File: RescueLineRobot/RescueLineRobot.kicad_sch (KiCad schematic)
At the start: 11 parts, among them J1 Conn_01x11, J2 Switch, J3 Motor 1, J4 Motor 2, J5 Convertidor, J6 Laser 1, J7 Laser 2, J8 Laser 3, J9 Bateria, U1 ROB-14450, U2 ESP32-DEVKIT-V1

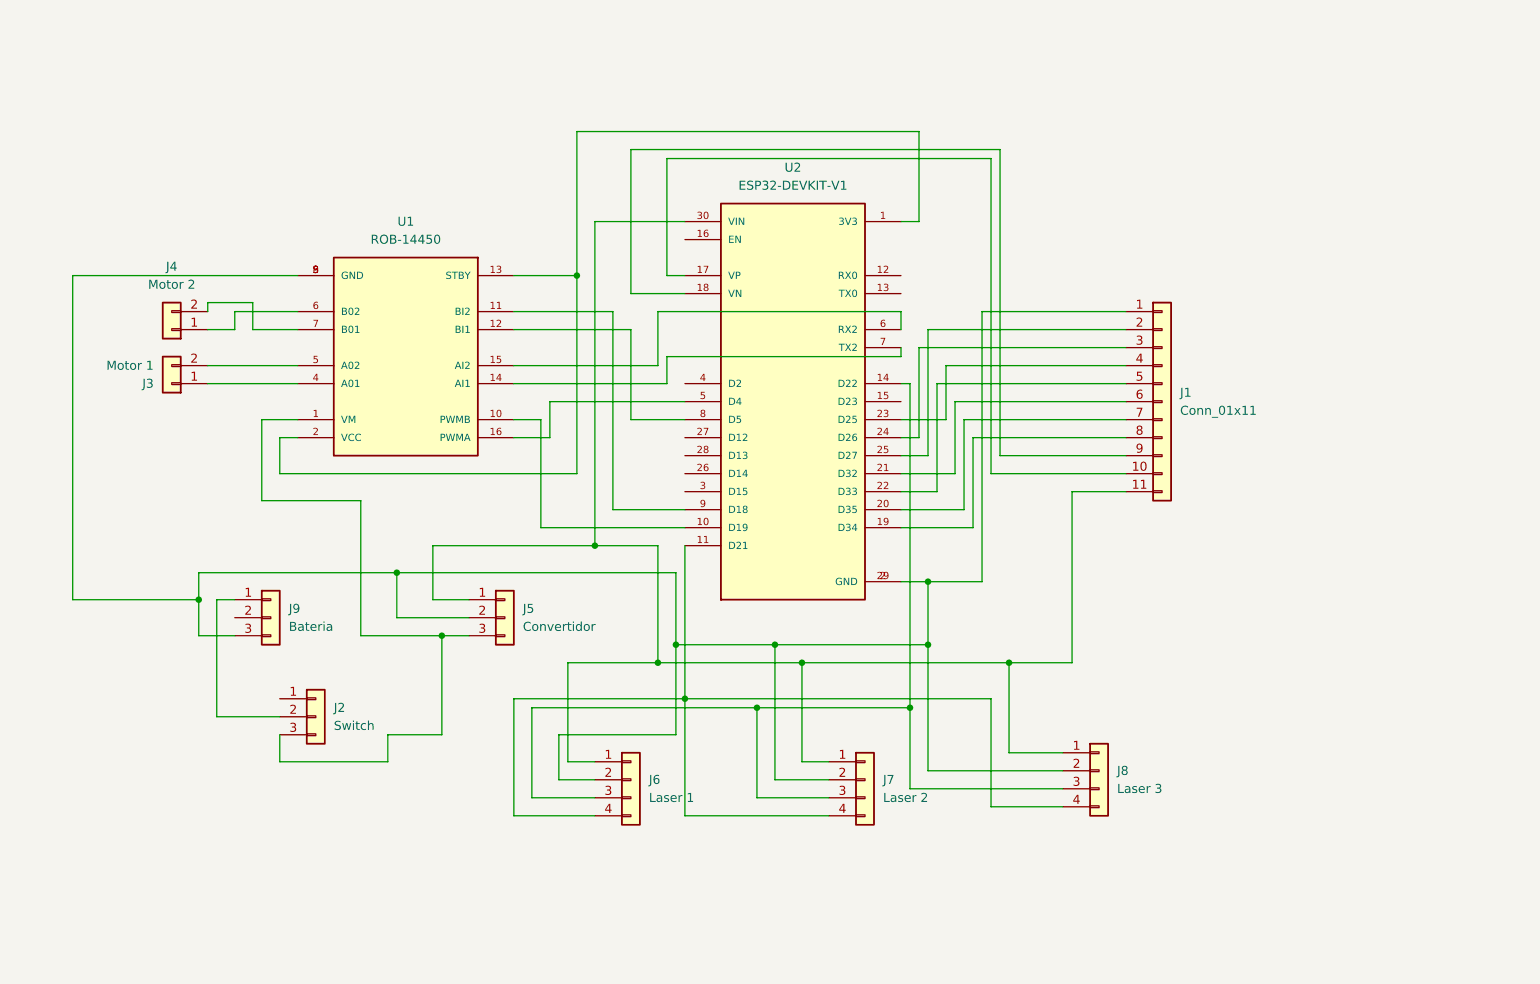
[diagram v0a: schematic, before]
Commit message: Boton y encoders
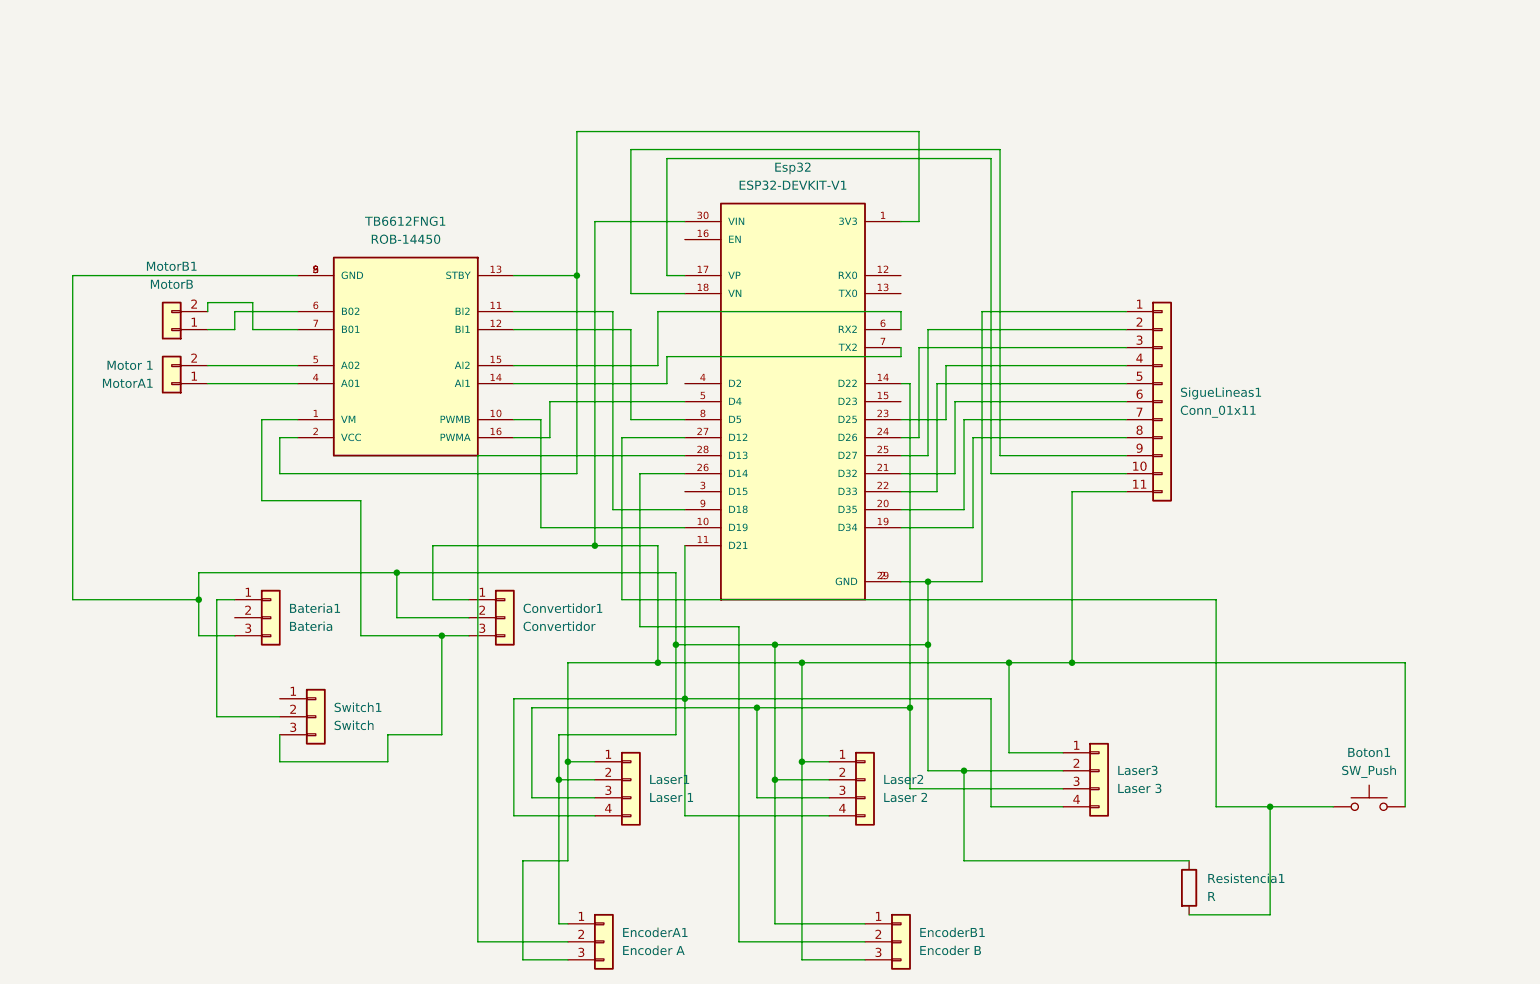
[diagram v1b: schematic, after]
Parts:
- added Boton1: SW_Push, Button_Switch_THT:SW_PUSH-12mm, symbol Switch:SW_Push
- added EncoderA1: Encoder A, Connector_JST:JST_XA_B03B-XASK-1_1x03_P2.50mm_Vertical, symbol Connector_Generic:Conn_01x03
- added EncoderB1: Encoder B, Connector_JST:JST_XA_B03B-XASK-1_1x03_P2.50mm_Vertical, symbol Connector_Generic:Conn_01x03
- added Resistencia1: R, Resistor_THT:R_Axial_DIN0617_L17.0mm_D6.0mm_P25.40mm_Horizontal, symbol Device:R
- MotorB1: renamed from J4; value Motor 2 -> MotorB
- renumbered J9 to Bateria1, J5 to Convertidor1, U2 to Esp32, J6 to Laser1, J7 to Laser2, J8 to Laser3, J3 to MotorA1, J1 to SigueLineas1, J2 to Switch1, U1 to TB6612FNG1
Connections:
- net at Convertidor1.1 (Pin_1), Esp32.30 (VIN), Laser1.1 (Pin_1)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: now also Boton1.2, EncoderA1.3 (Pin_3), EncoderB1.3 (Pin_3)
- net at Bateria1.3 (Pin_3), Convertidor1.2 (Pin_2), Esp32.2 (GND)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: now also EncoderA1.1 (Pin_1), EncoderB1.1 (Pin_1), Resistencia1.1
- net at Esp32.26 (D14): now also EncoderB1.2 (Pin_2)
- net at Esp32.27 (D12): now also Boton1.1, Resistencia1.2
- net at Esp32.28 (D13): now also EncoderA1.2 (Pin_2)

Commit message: Estamos Casi
Están todas las rutas hechas, todos los puertos necesarios, sólo falta nombrar al robot y poner gráficas
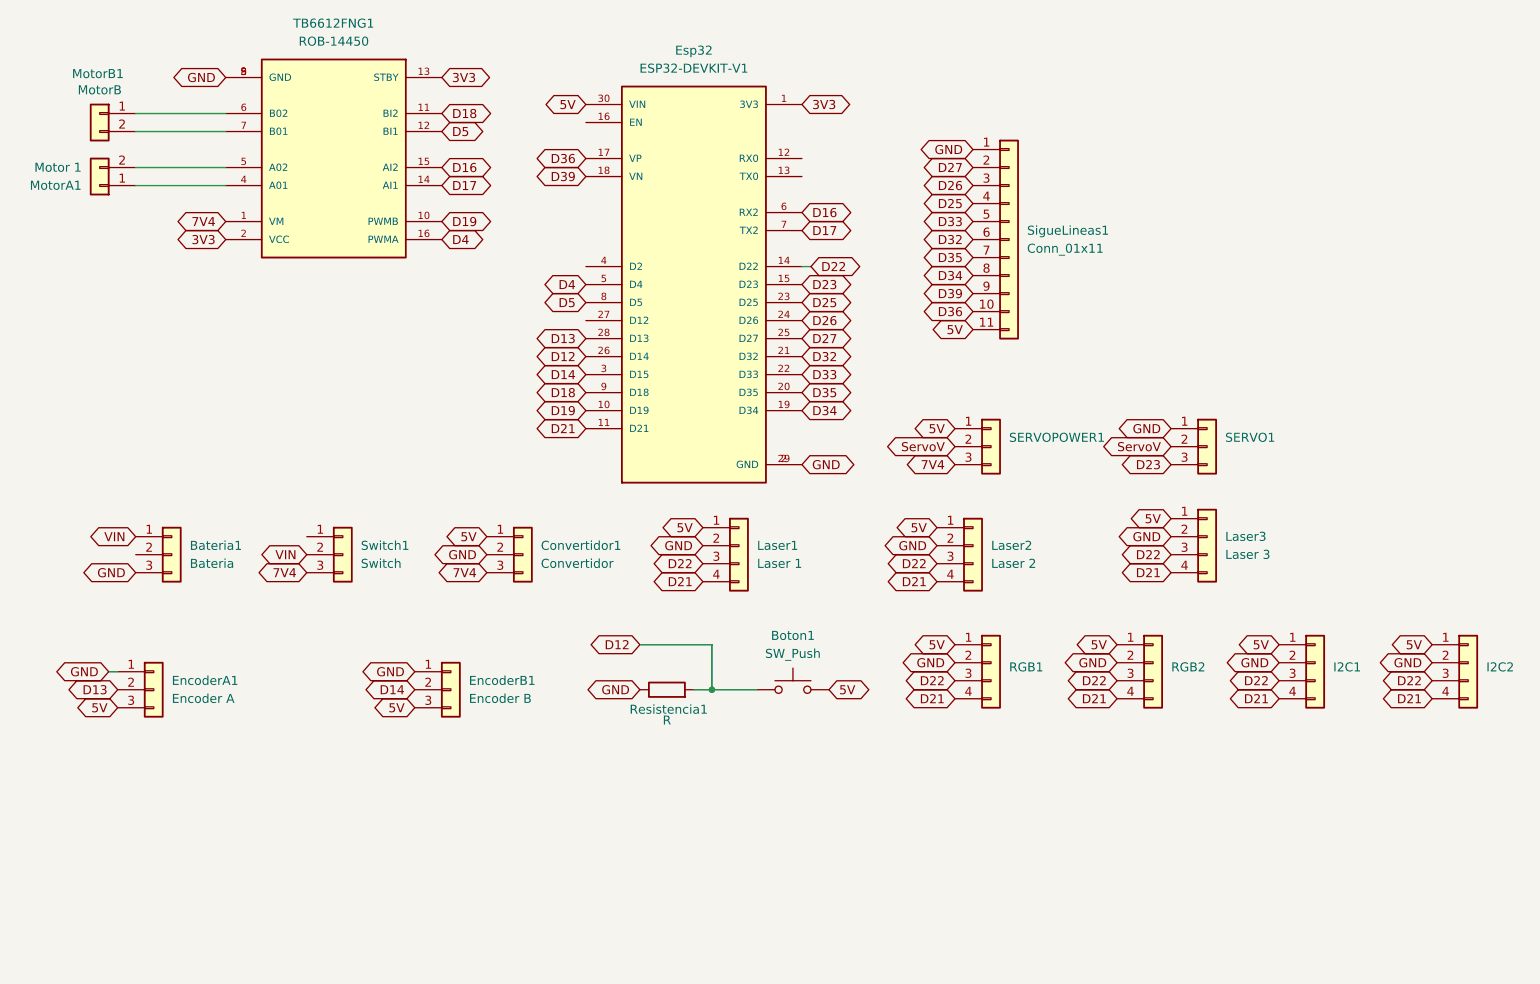
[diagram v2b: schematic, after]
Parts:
- added I2C1, I2C2, RGB1, RGB2: ~, Connector_JST:JST_XH_B4B-XH-A_1x04_P2.50mm_Vertical, symbol Connector_Generic:Conn_01x04
- added SERVO1: Conn_01x03, Connector_JST:JST_XH_B3B-XH-A_1x03_P2.50mm_Vertical, symbol Connector_Generic:Conn_01x03
- added SERVOPOWER1: Conn_01x03, Connector_PinHeader_1.27mm:PinHeader_1x03_P1.27mm_Vertical, symbol Connector_Generic:Conn_01x03
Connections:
- net 5V: now reaches Boton1.2, Convertidor1.1 (Pin_1), EncoderA1.3 (Pin_3), EncoderB1.3 (Pin_3), Esp32.30 (VIN), Laser1.1 (Pin_1), Laser2.1 (Pin_1), Laser3.1 (Pin_1), SigueLineas1.11 (Pin_11)
- net 5V: now also I2C1.1 (Pin_1), I2C2.1 (Pin_1), RGB1.1 (Pin_1), RGB2.1 (Pin_1), SERVOPOWER1.1 (Pin_1)
- net GND: now reaches Bateria1.3 (Pin_3), Convertidor1.2 (Pin_2), EncoderA1.1 (Pin_1), EncoderB1.1 (Pin_1), Esp32.2 (GND), Esp32.29 (GND), Laser1.2 (Pin_2), Laser2.2 (Pin_2), Laser3.2 (Pin_2), Resistencia1.1, SigueLineas1.1 (Pin_1), TB6612FNG1.3 (GND), TB6612FNG1.8 (GND), TB6612FNG1.9 (GND)
- net GND: now also I2C1.2 (Pin_2), I2C2.2 (Pin_2), RGB1.2 (Pin_2), RGB2.2 (Pin_2), SERVO1.1 (Pin_1)
- net D22: now reaches Esp32.14 (D22), Laser1.3 (Pin_3), Laser2.3 (Pin_3), Laser3.3 (Pin_3)
- net D22: now also I2C1.3 (Pin_3), I2C2.3 (Pin_3), RGB1.3 (Pin_3), RGB2.3 (Pin_3)
- net D21: now reaches Esp32.11 (D21), Laser1.4 (Pin_4), Laser2.4 (Pin_4), Laser3.4 (Pin_4)
- net D21: now also I2C1.4 (Pin_4), I2C2.4 (Pin_4), RGB1.4 (Pin_4), RGB2.4 (Pin_4)
- net 7V4: now reaches Convertidor1.3 (Pin_3), Switch1.3 (Pin_3), TB6612FNG1.1 (VM)
- net 7V4: now also SERVOPOWER1.3 (Pin_3)
- net D19: now reaches Esp32.10 (D19), TB6612FNG1.10 (PWMB)
- net D18: now reaches Esp32.9 (D18), TB6612FNG1.11 (BI2)
- net D5: now reaches Esp32.8 (D5), TB6612FNG1.12 (BI1)
- net 3V3: now reaches Esp32.1 (3V3), TB6612FNG1.13 (STBY), TB6612FNG1.2 (VCC)
- net D17: now reaches Esp32.7 (TX2), TB6612FNG1.14 (AI1)
- net D16: now reaches Esp32.6 (RX2), TB6612FNG1.15 (AI2)
- net D4: now reaches Esp32.5 (D4), TB6612FNG1.16 (PWMA)
- net D12: now reaches Boton1.1, Resistencia1.2
- net D12: now also Esp32.26 (D14); no longer Esp32.27 (D12)
- net VIN: now reaches Bateria1.1 (Pin_1), Switch1.2 (Pin_2)
- net D14: now reaches EncoderB1.2 (Pin_2)
- net D14: now also Esp32.3 (D15); no longer Esp32.26 (D14)
- net D23: now reaches Esp32.15 (D23)
- net D23: now also SERVO1.3 (Pin_3)
- net D36: now reaches Esp32.17 (VP), SigueLineas1.10 (Pin_10)
- net D39: now reaches Esp32.18 (VN), SigueLineas1.9 (Pin_9)
- net D34: now reaches Esp32.19 (D34), SigueLineas1.8 (Pin_8)
- net D35: now reaches Esp32.20 (D35), SigueLineas1.7 (Pin_7)
- net D32: now reaches Esp32.21 (D32), SigueLineas1.6 (Pin_6)
- net D33: now reaches Esp32.22 (D33), SigueLineas1.5 (Pin_5)
- net D25: now reaches Esp32.23 (D25), SigueLineas1.4 (Pin_4)
- net D26: now reaches Esp32.24 (D26), SigueLineas1.3 (Pin_3)
- net D27: now reaches Esp32.25 (D27), SigueLineas1.2 (Pin_2)
- net D13: now reaches EncoderA1.2 (Pin_2), Esp32.28 (D13)
- new net ServoV: SERVO1.2 (Pin_2), SERVOPOWER1.2 (Pin_2)
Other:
- moved on the sheet: Bateria1, Boton1, Convertidor1, EncoderA1, EncoderB1, Esp32, Laser1, Laser2, Laser3, MotorA1, MotorB1, Resistencia1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

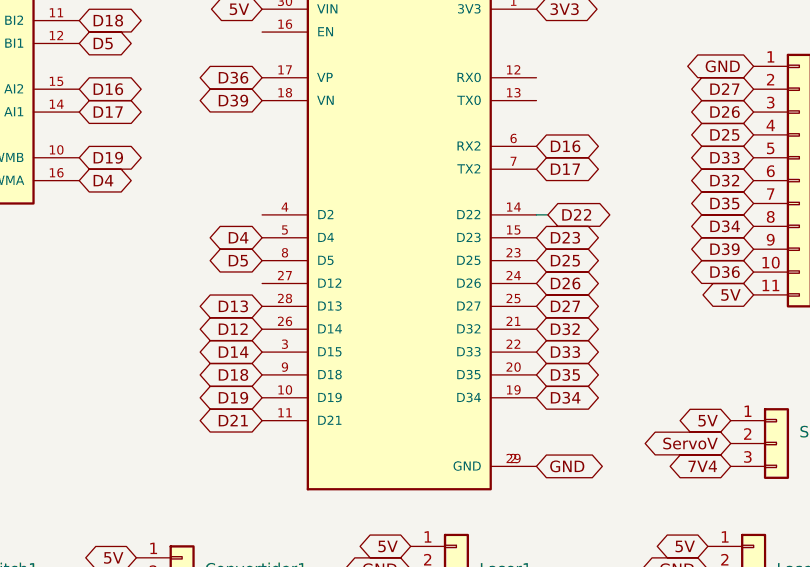
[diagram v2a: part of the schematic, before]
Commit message: Dynamis a nacido
Estamos listos señores!!!
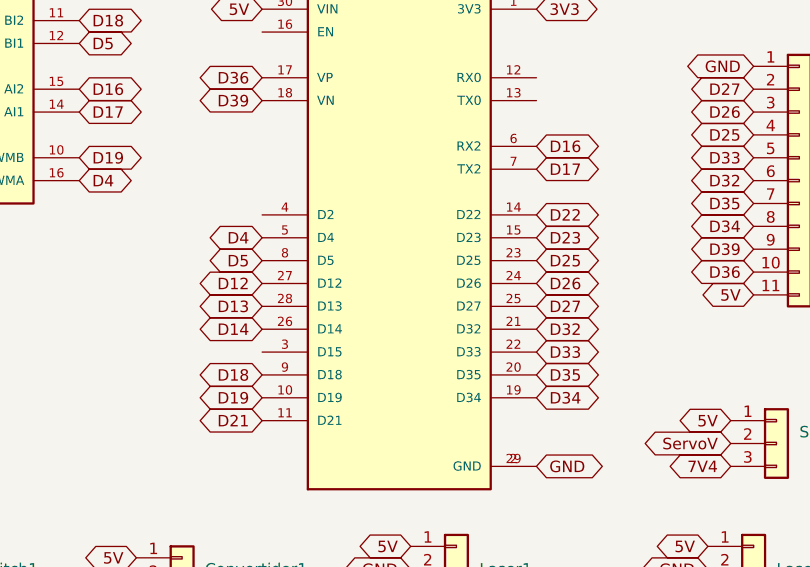
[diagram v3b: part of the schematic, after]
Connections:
- net D12: now also Esp32.27 (D12); no longer Esp32.26 (D14)
- net D14: now also Esp32.26 (D14); no longer Esp32.3 (D15)
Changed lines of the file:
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@@
-	(wire
-		(pts
-			(xy 125.73 53.34) (xy 127 53.34)
-		)
-		(stroke
-			(width 0)
-			(type default)
-		)
-	)
 	(wire
 		(pts
@@
 	(global_label "D14"
 		(shape bidirectional)
-		(at 95.25 68.58 180)
-		(fields_autoplaced yes)
-		(effects
-			(font
-				(size 1.27 1.27)
-			)
-			(justify right)
-		)
-		(property "Intersheetrefs" "${INTERSHEET_REFS}"
-			(at 87.4645 68.58 0)
+		(at 95.25 66.04 180)
+		(fields_autoplaced yes)
+		(effects
+			(font
+				(size 1.27 1.27)
+			)
+			(justify right)
+		)
+		(property "Intersheetrefs" "${INTERSHEET_REFS}"
+			(at 87.4645 66.04 0)
 			(effects
 				(font
@@
 	(global_label "D22"
 		(shape bidirectional)
-		(at 127 53.34 0)
+		(at 125.73 53.34 0)
 		(fields_autoplaced yes)
 		(effects
@@
 		)
 		(property "Intersheetrefs" "${INTERSHEET_REFS}"
-			(at 134.7855 53.34 0)
+			(at 133.5155 53.34 0)
 			(effects
 				(font
@@
 	(global_label "D12"
 		(shape bidirectional)
-		(at 95.25 66.04 180)
-		(fields_autoplaced yes)
-		(effects
-			(font
-				(size 1.27 1.27)
-			)
-			(justify right)
-		)
-		(property "Intersheetrefs" "${INTERSHEET_REFS}"
-			(at 87.4645 66.04 0)
-			(effects
-				(font
+		(at 95.25 60.96 180)
+		(fields_autoplaced yes)
+		(effects
+			(font
+				(size 1.27 1.27)
+			)
+			(justify right)
+		)
+		(property "Intersheetrefs" "${INTERSHEET_REFS}"
+			(at 87.4645 60.96 0)
+			(effects
+				(font
